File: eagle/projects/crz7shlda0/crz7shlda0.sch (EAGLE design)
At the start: 27 parts, among them J1 HDR-2X8, Q1 BSS138, Q5 BSS138, Q6 BSS138, T1 MMBT3904

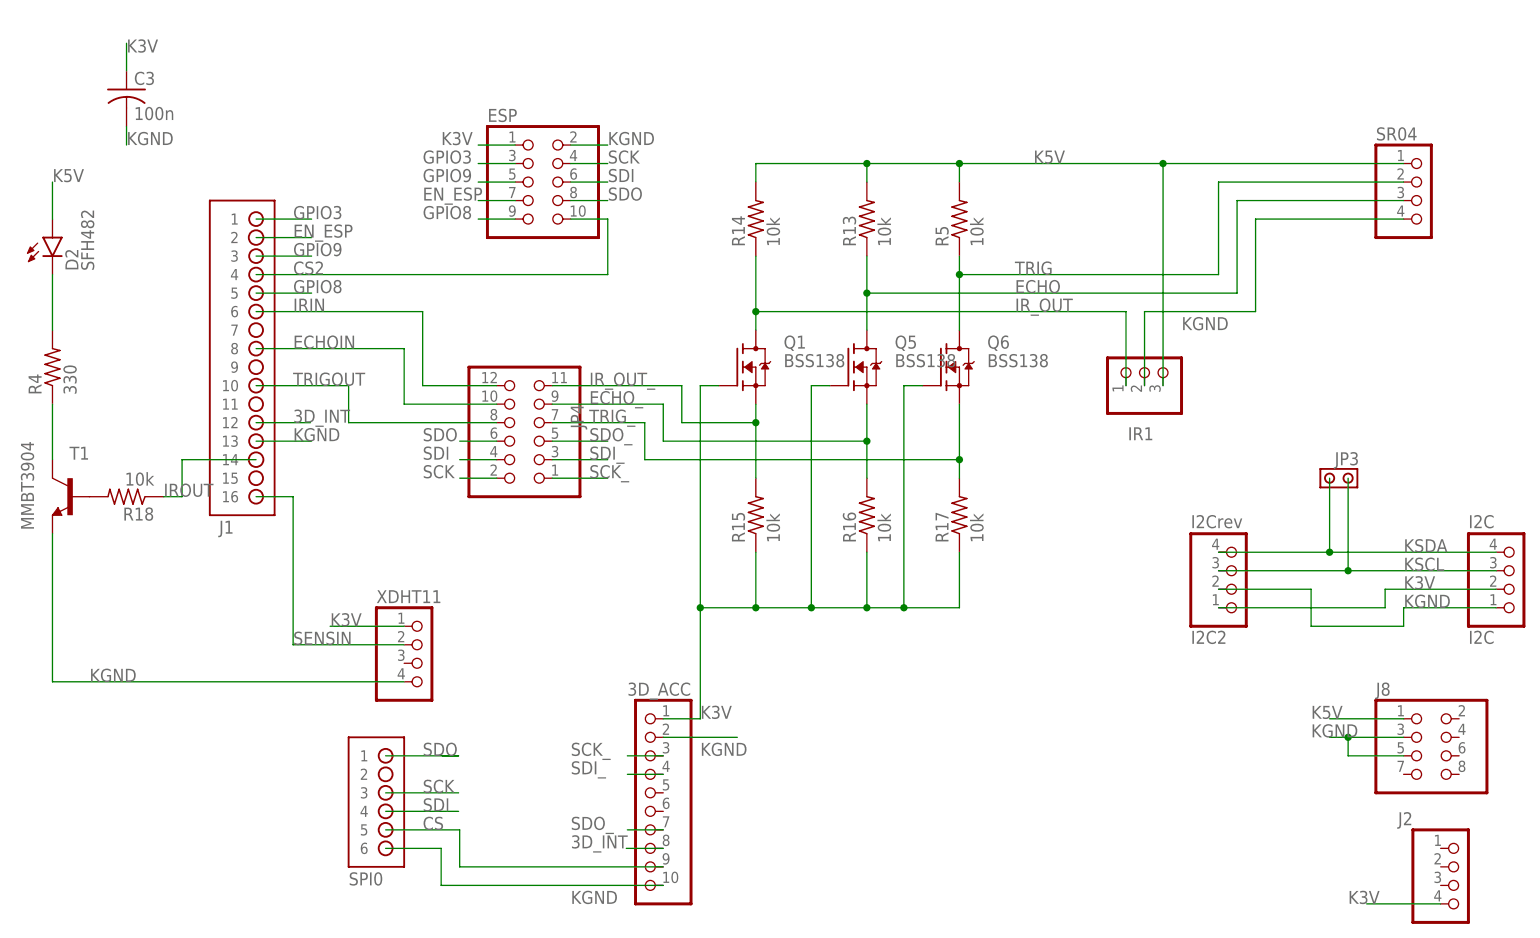
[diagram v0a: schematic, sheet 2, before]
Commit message: just push latest hanging changes to repo
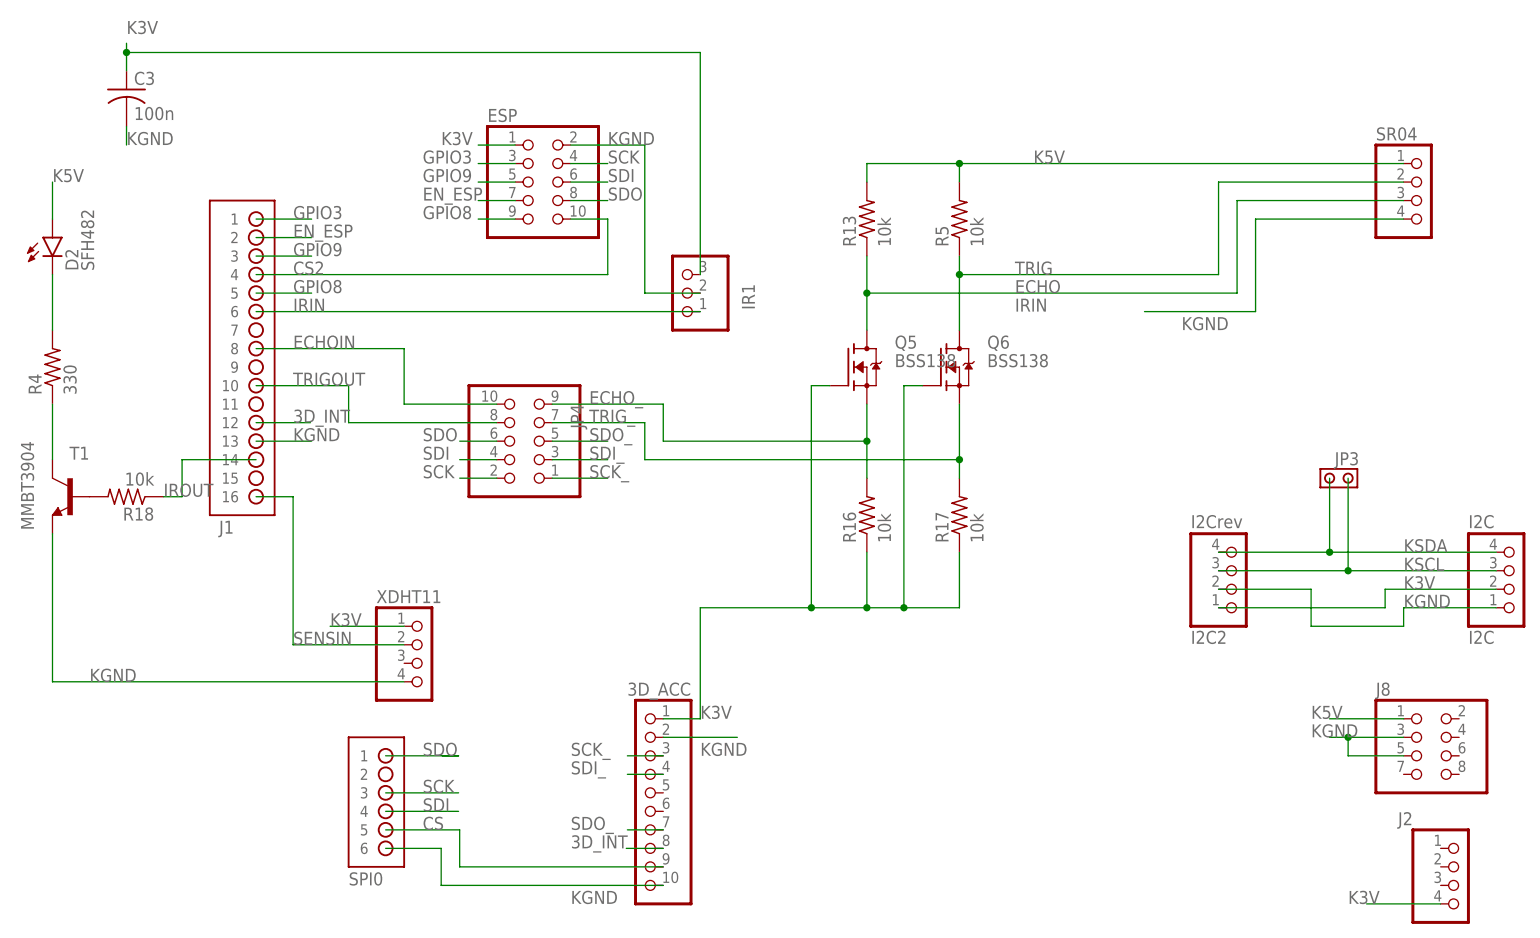
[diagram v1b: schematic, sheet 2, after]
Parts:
- removed Q1: BSS138, bss138_10:BSS138
- removed R14, R15: 10k, rcl:R-US_R0402
- JP4: device pinhead:PINHD-2X6 -> pinhead:PINHD-2X5
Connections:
- removed net IR_OUT: IR1.1, Q1.D, R14.1
- removed net IR_OUT_: JP4.11, Q1.S, R15.2
- net IRIN: now also IR1.1; no longer JP4.12
- net K3V: now also IR1.3; no longer Q1.G, R15.1
- net K5V: no longer IR1.3, R14.2
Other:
- moved on the sheet: IR1
